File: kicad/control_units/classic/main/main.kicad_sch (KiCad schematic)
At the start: 12 parts, among them J1 Conn_01x05, J2 USB_C_Receptacle_USB2.0_14P, U1 STM32U031F4Px, U2 AZ1117CH2-3.3

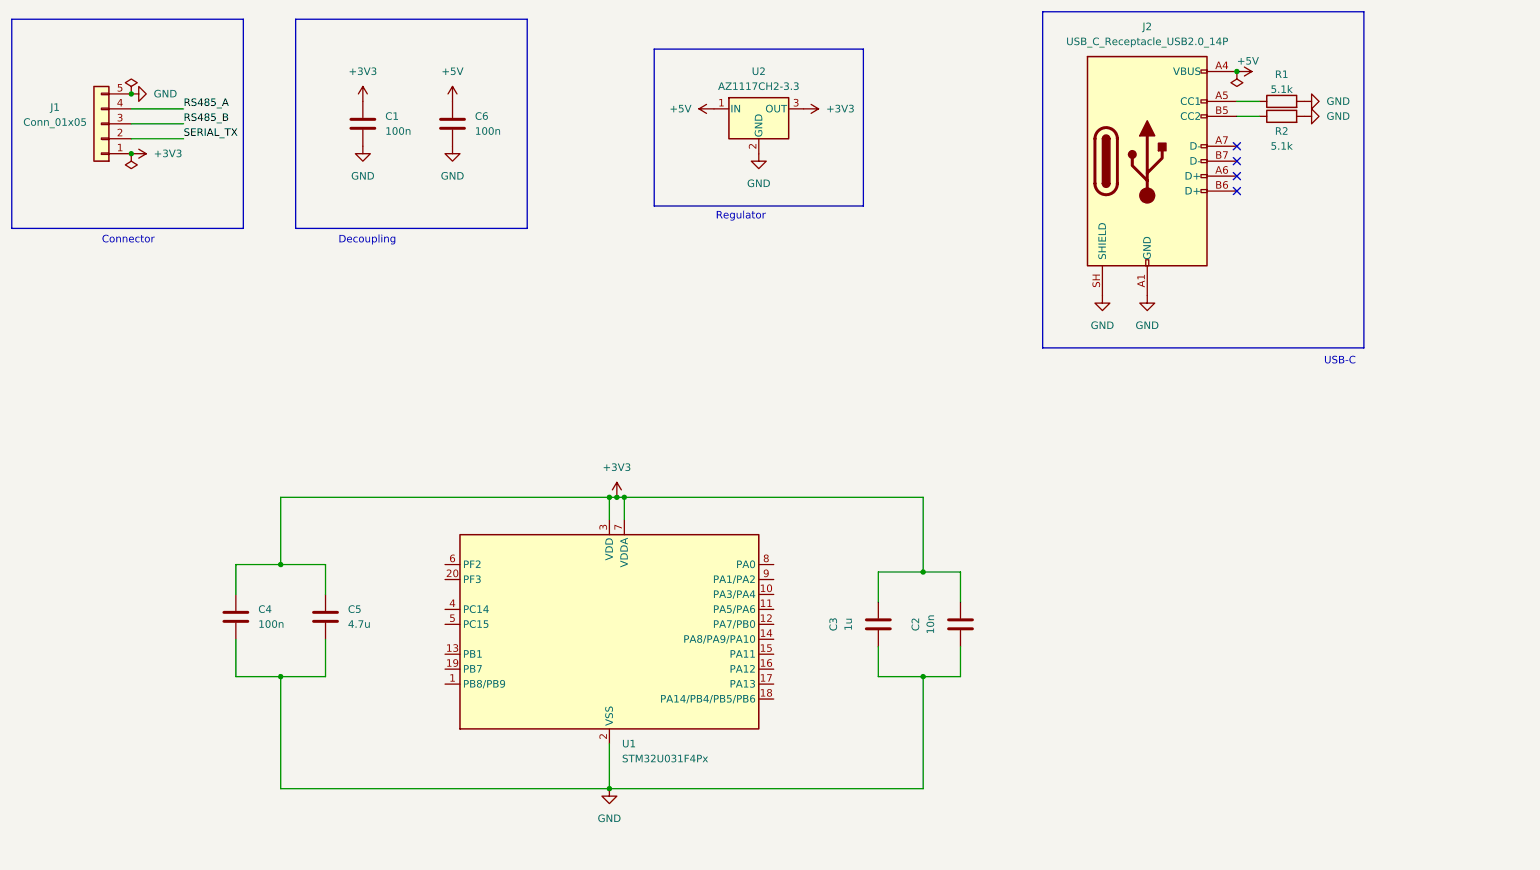
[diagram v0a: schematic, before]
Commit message: More stuff for Classic control unit
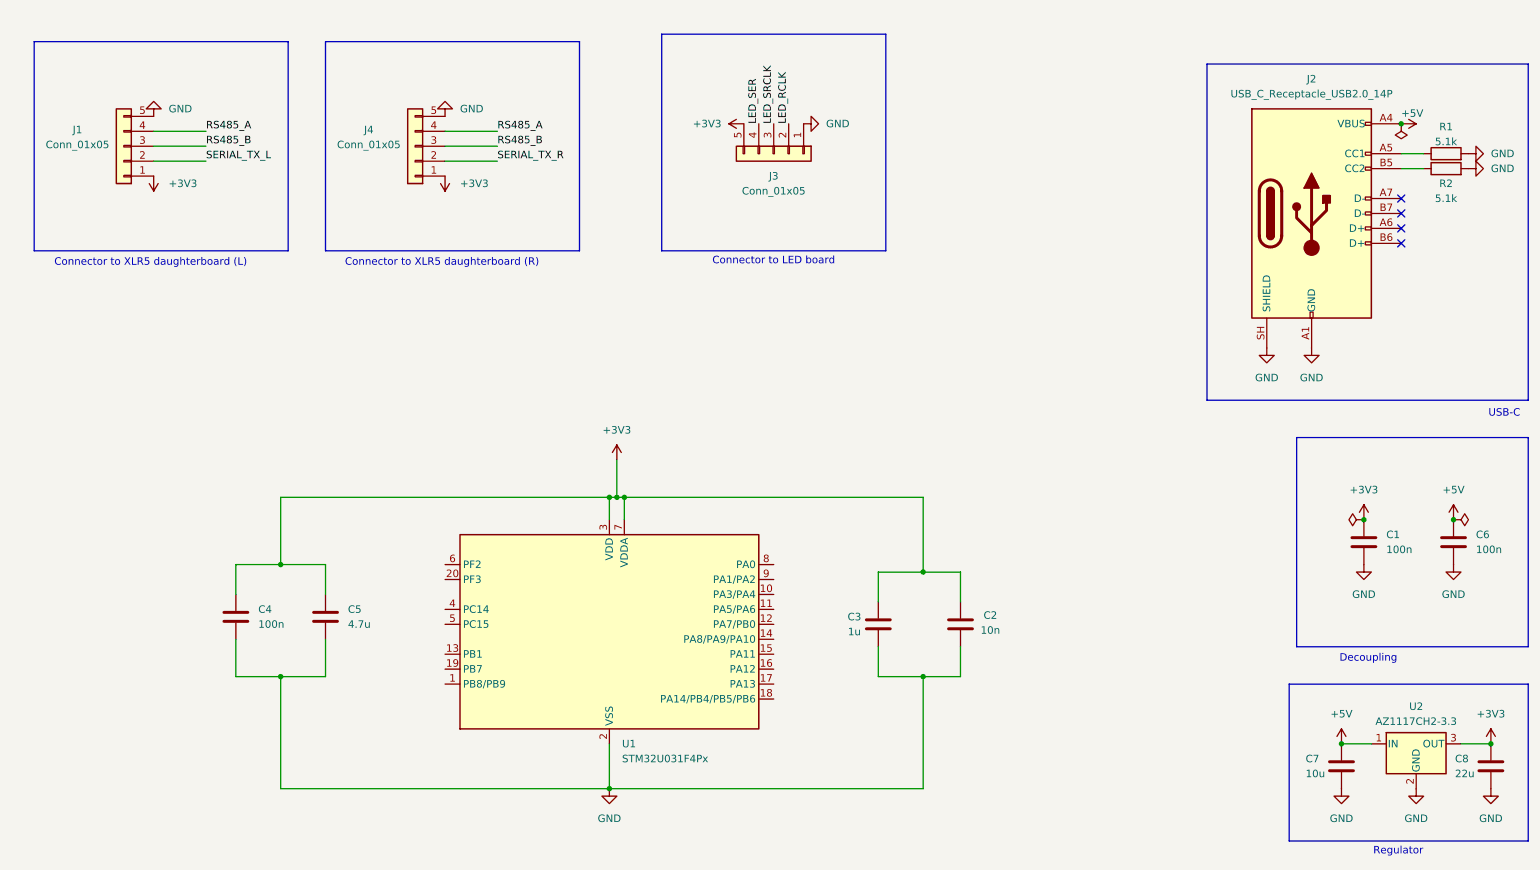
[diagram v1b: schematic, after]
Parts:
- added C7: 10u, symbol Device:C
- added C8: 22u, symbol Device:C
- added J3, J4: Conn_01x05, symbol Connector_Generic:Conn_01x05
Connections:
- net +3V3: now also C8.2, J3.5 (Pin_5), J4.1 (Pin_1)
- net +5V: now also C7.2
- net GND: now also C7.1, C8.1, J3.1 (Pin_1), J4.5 (Pin_5)
- net RS485_A: now also J4.4 (Pin_4)
- net RS485_B: now also J4.3 (Pin_3)
- net SERIAL_TX renamed SERIAL_TX_L
- new net LED_RCLK: J3.2 (Pin_2)
- new net LED_SER: J3.4 (Pin_4)
- new net LED_SRCLK: J3.3 (Pin_3)
- new net SERIAL_TX_R: J4.2 (Pin_2)
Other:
- note added: "Connector to LED board"
- note added: "Connector to XLR5 daughterboard (L)"
- note added: "Connector to XLR5 daughterboard (R)"
- note removed: "Connector"
- moved on the sheet: C1, C6, J1, J2, R1, R2, U2
